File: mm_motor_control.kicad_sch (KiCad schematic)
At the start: 0 parts

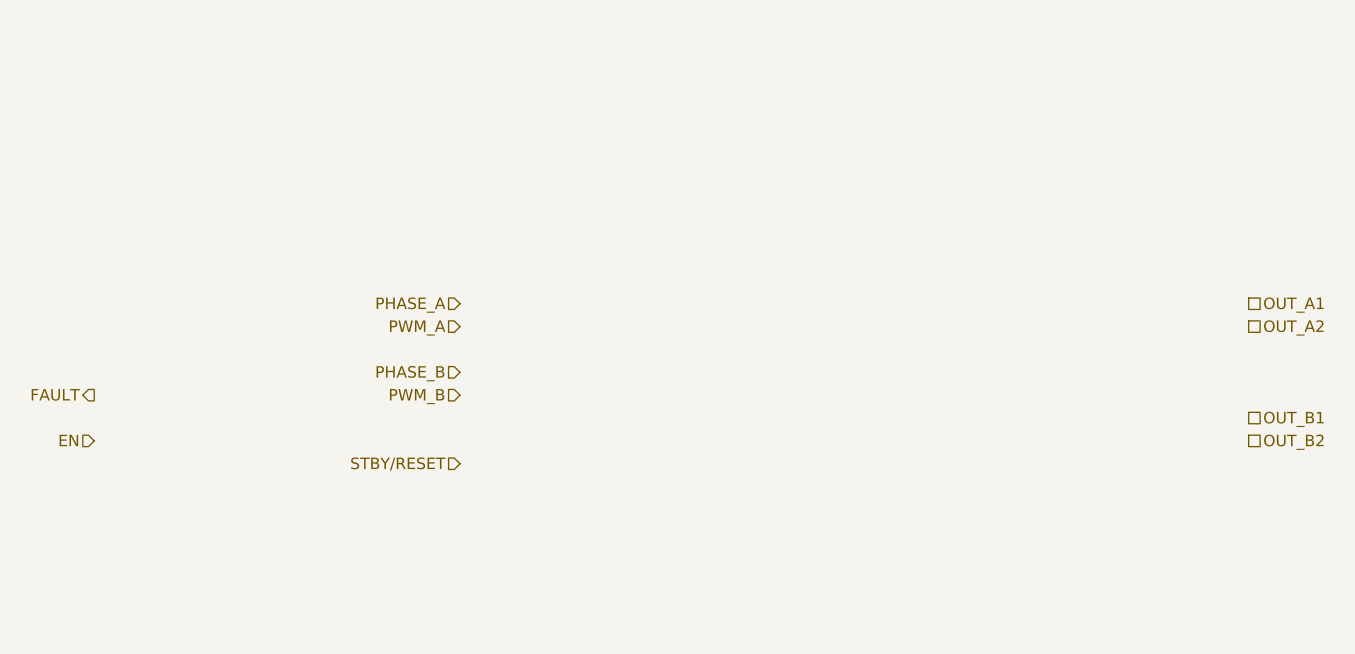
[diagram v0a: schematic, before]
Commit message: tp2
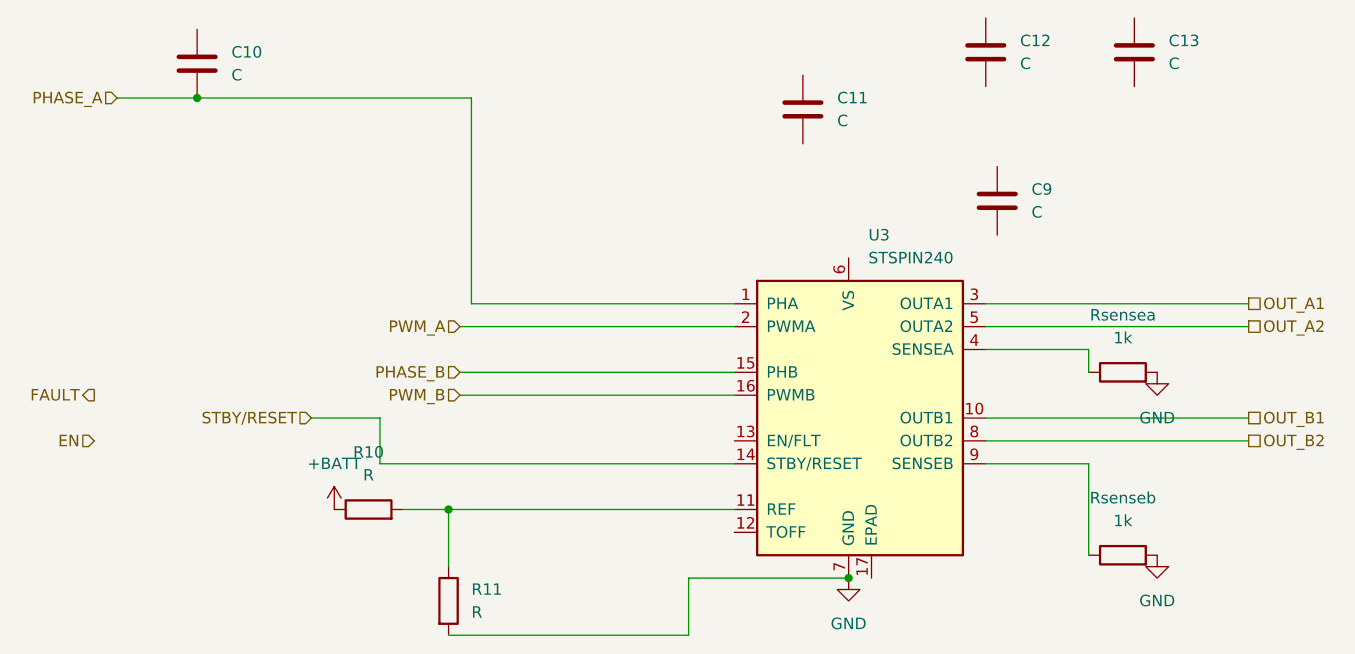
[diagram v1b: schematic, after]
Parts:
- added C10, C11, C12, C13, C9: C, symbol Device:C
- added R10, R11: R, symbol Device:R
- added Rsensea, Rsenseb: 1k, symbol Device:R
- added U3: STSPIN240, Package_DFN_QFN:VQFN-16-1EP_3x3mm_P0.5mm_EP1.8x1.8mm, symbol Driver_Motor:STSPIN240
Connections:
- net OUT_A1: now also U3.3 (OUTA1)
- net OUT_A2: now also U3.5 (OUTA2)
- net OUT_B1: now also U3.10 (OUTB1)
- net OUT_B2: now also U3.8 (OUTB2)
- net PHASE_A: now also C10.2, U3.1 (PHA)
- net PHASE_B: now also U3.15 (PHB)
- net PWM_A: now also U3.2 (PWMA)
- net PWM_B: now also U3.16 (PWMB)
- net STBY/RESET: now also U3.14 (STBY/RESET)
- new net: R10.2, R11.1, U3.11 (REF)
- new net: Rsensea.1, U3.4 (SENSEA)
- new net: Rsenseb.1, U3.9 (SENSEB)
- new net +BATT: R10.1
- new net GND: R11.2, Rsensea.2, Rsenseb.2, U3.7 (GND)
